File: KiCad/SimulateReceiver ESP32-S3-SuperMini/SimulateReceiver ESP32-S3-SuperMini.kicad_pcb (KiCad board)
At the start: 4 copper layers, 23.5 x 18 mm, 13 parts, among them IC1 CD4021BM96, J1 Conn_01x09, J2 Conn_01x09, J3 Conn_Coaxial, J4 Conn_01x06, U1 LM1881M, U2 ESP32-DevKitC

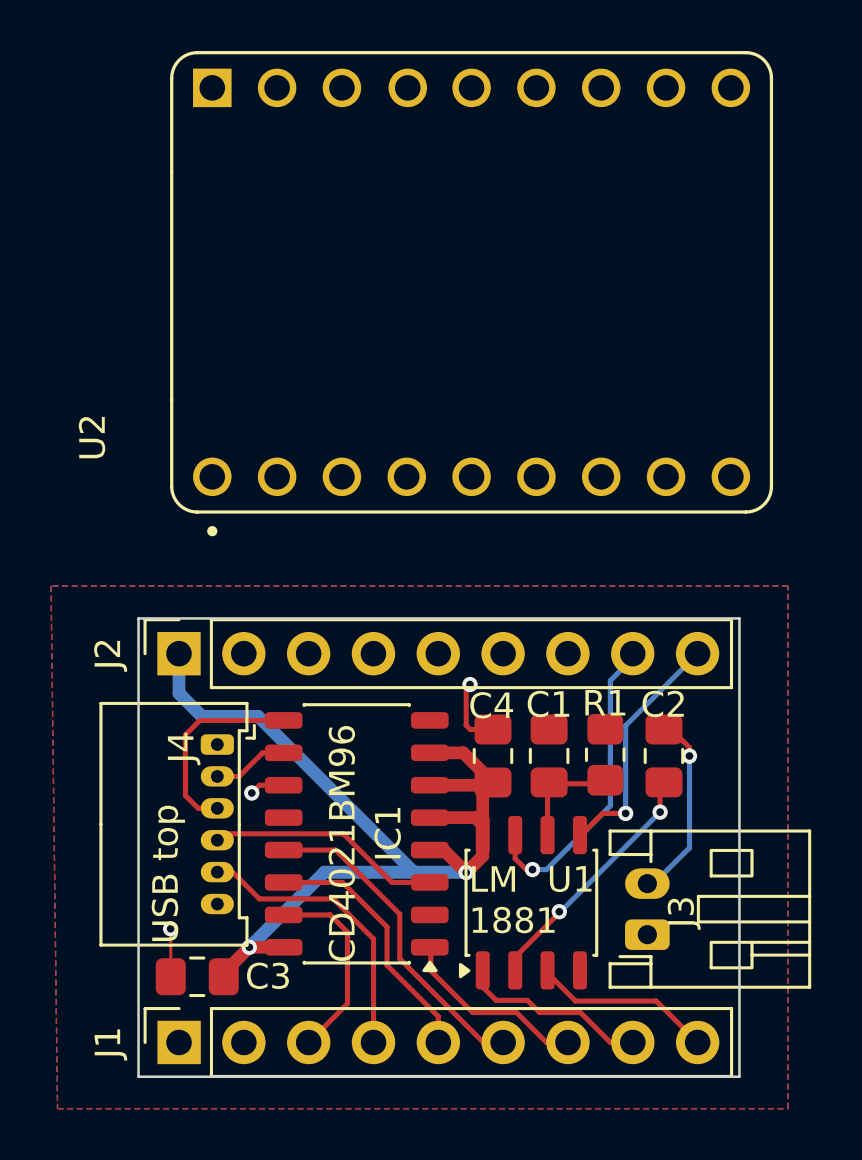
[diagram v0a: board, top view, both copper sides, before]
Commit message: Add files via upload
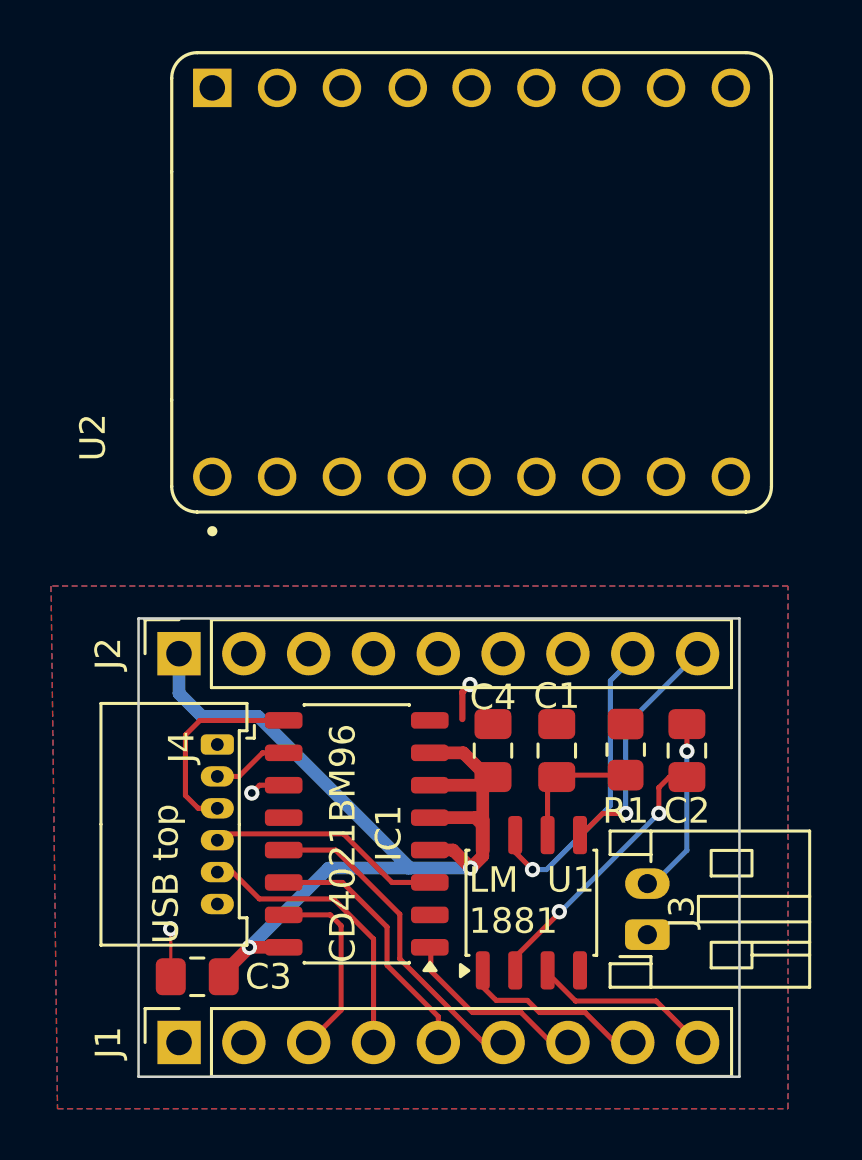
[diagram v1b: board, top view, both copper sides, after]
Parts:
- moved C2 0.92 mm to (123.9, 87.2)
- moved R1 0.82 mm to (121.5, 87.2)
- moved C1 0.37 mm to (118.8, 87.2)
- moved C4 0.21 mm to (116.3, 87.2)
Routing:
- net GND: track 6.23 -> 4.92 mm
- net Net-(U1-RSET): track 4.27 -> 4.84 mm
